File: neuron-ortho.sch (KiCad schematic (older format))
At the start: 138 parts, among them J1 USB_C_Receptacle, J2 Conn_01x04_Male, J3 Conn_01x06_Male, J4 Conn_01x04_Male, J5 Conn_01x04_Male, Q1 DTC123J, SW1 SW_Push, U1 STM32F303C6Tx, U2 NCP1117-3.3_SOT223, U3 USBLC6-2SC6, Y1 8MHz

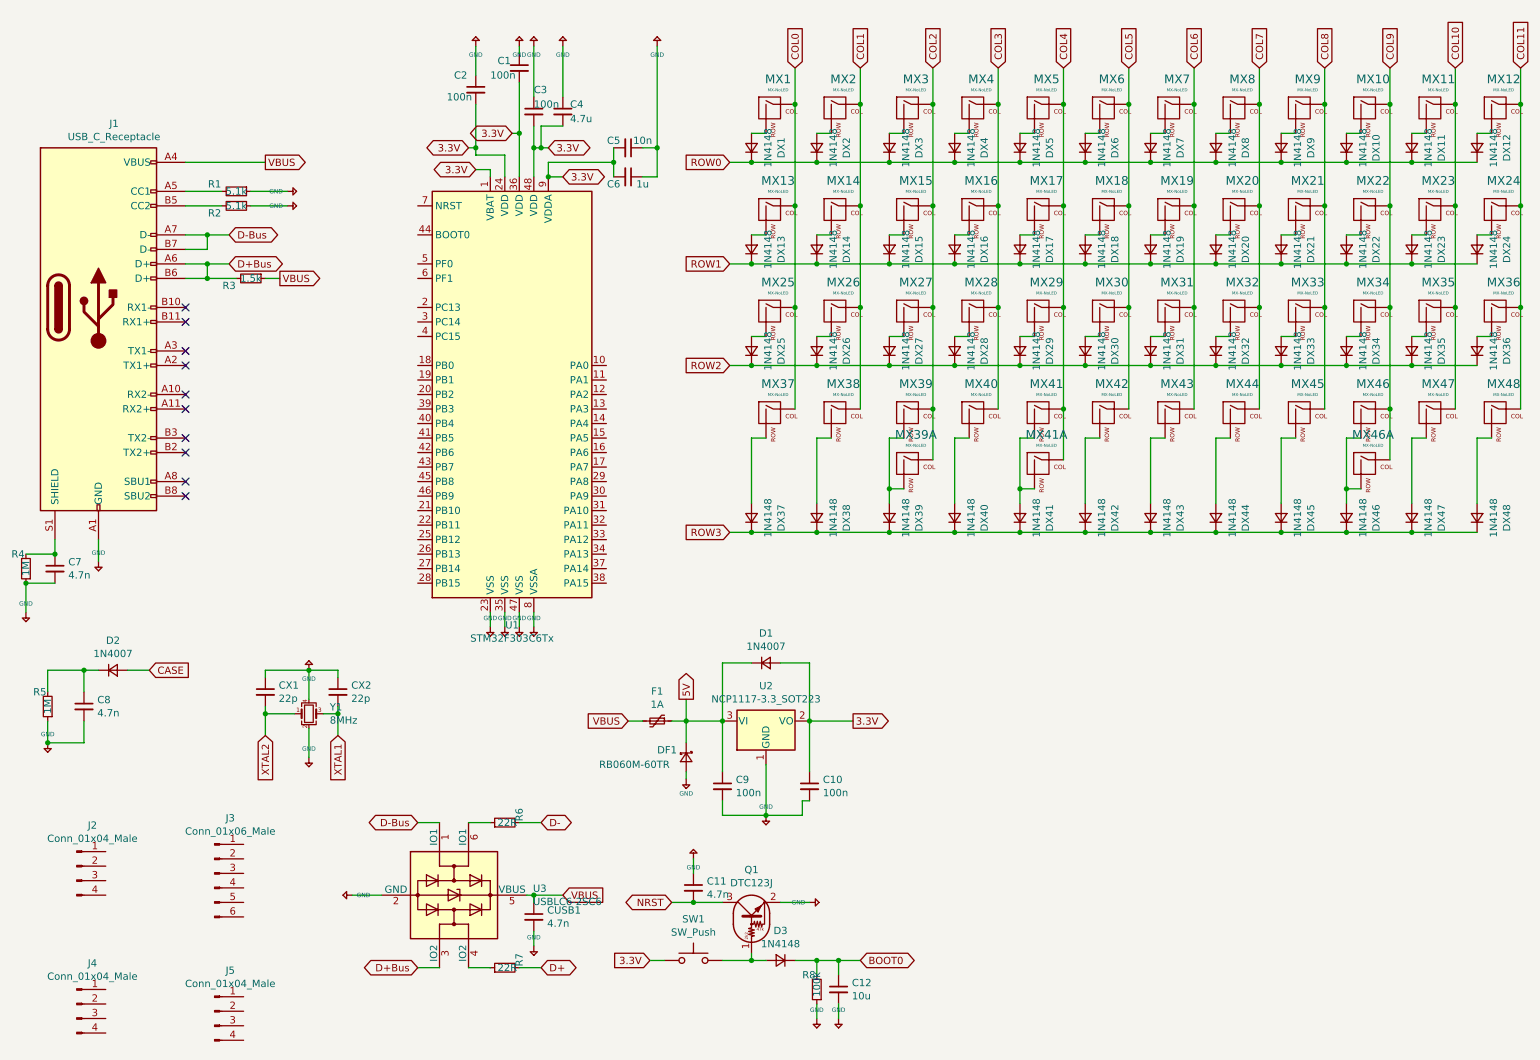
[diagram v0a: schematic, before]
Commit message: Assigned some MCU pins
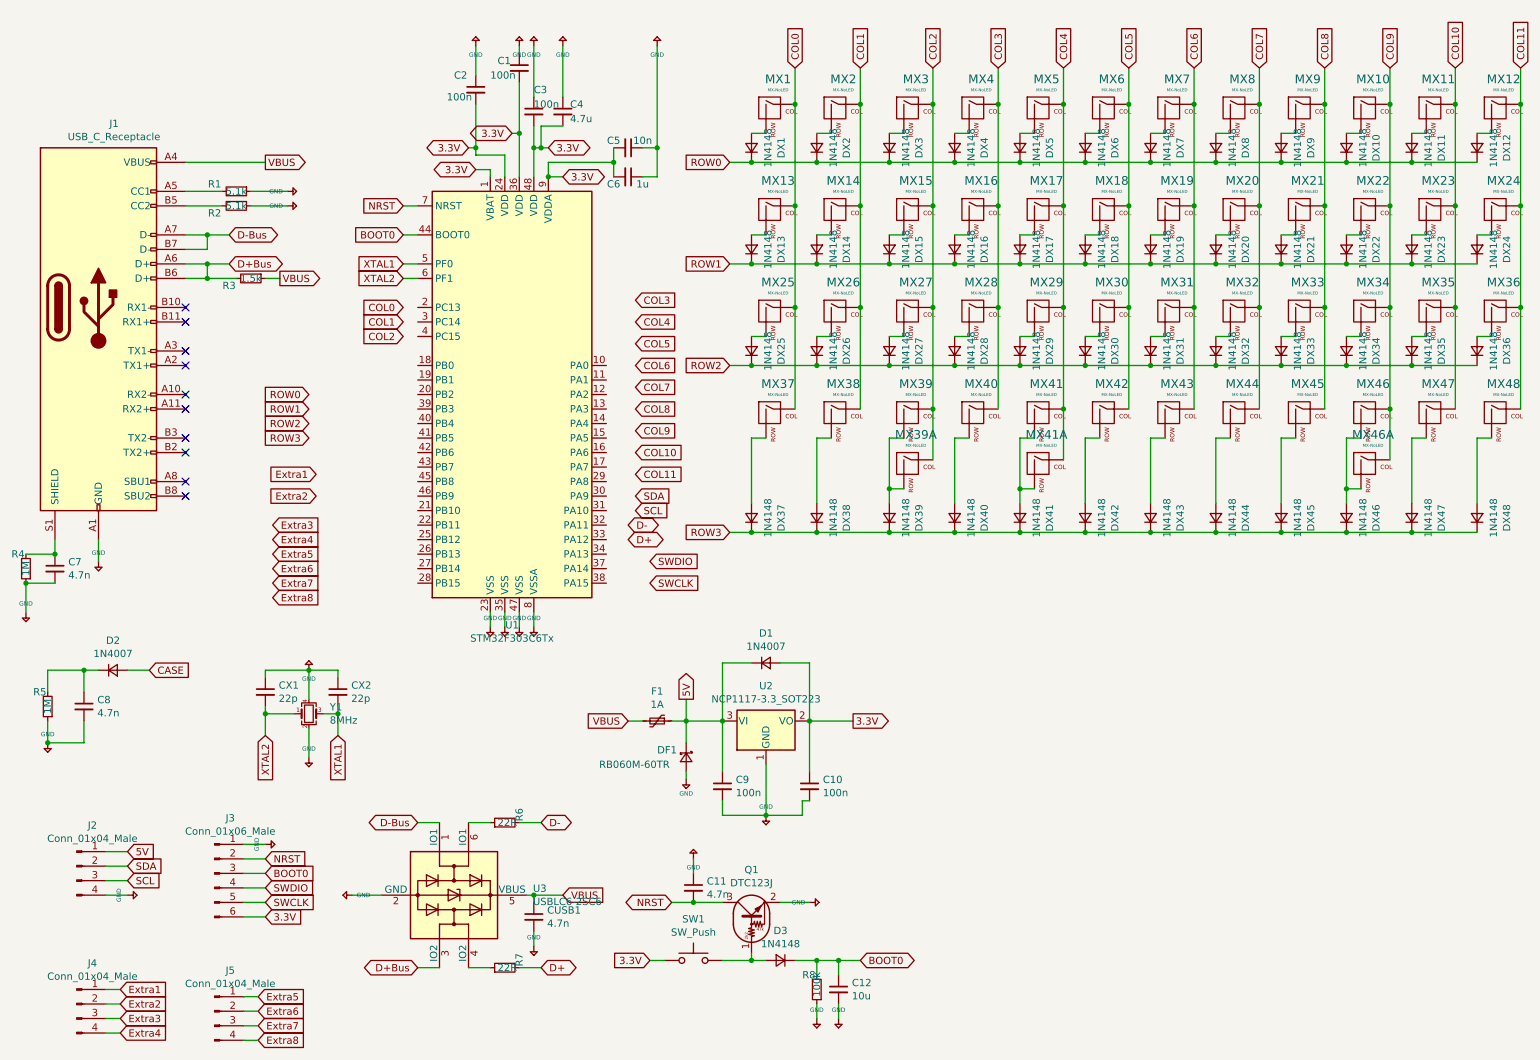
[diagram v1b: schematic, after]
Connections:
- net +5V: now also J2.4 (Pin_4), J3.1 (Pin_1)
- net 3.3V: now also J3.6 (Pin_6)
- net 5V: now also J2.1 (Pin_1)
- net BOOT0: now also J3.3 (Pin_3), U1.44 (BOOT0)
- net NRST: now also J3.2 (Pin_2), U1.7 (NRST)
- net XTAL1: now also U1.5 (PF0)
- net XTAL2: now also U1.6 (PF1)
- net SDA: now reaches J2.2 (Pin_2)
- net SCL: now reaches J2.3 (Pin_3)
- net SWDIO: now reaches J3.4 (Pin_4)
- net SWCLK: now reaches J3.5 (Pin_5)
- net Extra1: now reaches J4.1 (Pin_1)
- net Extra2: now reaches J4.2 (Pin_2)
- net Extra3: now reaches J4.3 (Pin_3)
- net Extra4: now reaches J4.4 (Pin_4)
- net Extra5: now reaches J5.1 (Pin_1)
- net Extra6: now reaches J5.2 (Pin_2)
- net Extra7: now reaches J5.3 (Pin_3)
- net Extra8: now reaches J5.4 (Pin_4)
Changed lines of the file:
@@
 Wire Wire Line
 	6600 2700 6700 2700
+Text GLabel 3250 1800 0    50   Input ~ 0
+NRST
+Wire Wire Line
+	3350 1800 3250 1800
+Wire Wire Line
+	3250 2000 3350 2000
+Text GLabel 3250 2200 0    50   Input ~ 0
+XTAL1
+Text GLabel 3250 2300 0    50   Input ~ 0
+XTAL2
+Wire Wire Line
+	3250 2200 3350 2200
+Wire Wire Line
+	3350 2300 3250 2300
+Text GLabel 4800 4000 2    50   BiDi ~ 0
+D-
+Text GLabel 4800 4100 2    50   BiDi ~ 0
+D+
+Text GLabel 3250 2500 0    50   Input ~ 0
+COL0
+Text GLabel 3250 2600 0    50   Input ~ 0
+COL1
+Text GLabel 3250 2700 0    50   Input ~ 0
+COL2
+Text GLabel 2600 3100 0    50   Input ~ 0
+ROW0
+Text GLabel 2600 3200 0    50   Input ~ 0
+ROW1
+Text GLabel 2600 3300 0    50   Input ~ 0
+ROW2
+Text GLabel 2600 3400 0    50   Input ~ 0
+ROW3
+Text GLabel 4850 2450 2    50   Input ~ 0
+COL3
+Text GLabel 4850 2600 2    50   Input ~ 0
+COL4
+Text GLabel 4850 2750 2    50   Input ~ 0
+COL5
+Text GLabel 4850 2900 2    50   Input ~ 0
+COL6
+Text GLabel 4850 3050 2    50   Input ~ 0
+COL7
+Text GLabel 4850 3200 2    50   Input ~ 0
+COL8
+Text GLabel 4850 3350 2    50   Input ~ 0
+COL9
+Text GLabel 4850 3500 2    50   Input ~ 0
+COL10
+Text GLabel 4850 3650 2    50   Input ~ 0
+COL11
+$Comp
+L keyboard_parts:GND #PWR?
+U 1 1 5E796914
+P 1350 6550
+F 0 "#PWR?" H 1350 6600 20  0001 C CNN
+F 1 "GND" H 1350 6609 30  0000 C CNN
+F 2 "" H 1350 6550 60  0000 C CNN
+F 3 "" H 1350 6550 60  0000 C CNN
+	1    1350 6550
+	0    -1   -1   0
+$EndComp
+$Comp
+L keyboard_parts:GND #PWR?
+U 1 1 5E79741B
+P 2300 6200
+F 0 "#PWR?" H 2300 6250 20  0001 C CNN
+F 1 "GND" H 2300 6259 30  0000 C CNN
+F 2 "" H 2300 6200 60  0000 C CNN
+F 3 "" H 2300 6200 60  0000 C CNN
+	1    2300 6200
+	0    -1   -1   0
+$EndComp
+Text GLabel 1350 6250 2    50   Input ~ 0
+5V
+Text GLabel 1350 6350 2    50   Input ~ 0
+SDA
+Text GLabel 1350 6450 2    50   Input ~ 0
+SCL
+Text GLabel 2300 6300 2    50   Input ~ 0
+NRST
+Text GLabel 2300 6400 2    50   Input ~ 0
+BOOT0
+Text GLabel 2300 6500 2    50   Input ~ 0
+SWDIO
+Text GLabel 2300 6600 2    50   Input ~ 0
+SWCLK
+Text GLabel 2300 6700 2    50   Input ~ 0
+3.3V
+Text GLabel 2250 7250 2    50   Input ~ 0
+Extra5
+Text GLabel 2250 7350 2    50   Input ~ 0
+Extra6
+Text GLabel 2250 7450 2    50   Input ~ 0
+Extra7
+Text GLabel 2250 7550 2    50   Input ~ 0
+Extra8
+Text GLabel 1300 7200 2    50   Input ~ 0
+Extra1
+Text GLabel 1300 7300 2    50   Input ~ 0
+Extra2
+Text GLabel 1300 7400 2    50   Input ~ 0
+Extra3
+Text GLabel 1300 7500 2    50   Input ~ 0
+Extra4
+Wire Wire Line
+	1200 6250 1350 6250
+Wire Wire Line
+	1200 6350 1350 6350
+Wire Wire Line
+	1200 6450 1350 6450
+Wire Wire Line
+	1200 6550 1350 6550
+Wire Wire Line
+	2150 6200 2300 6200
+Wire Wire Line
+	2150 6300 2300 6300
+Wire Wire Line
+	2150 6400 2300 6400
+Wire Wire Line
+	2150 6500 2300 6500
+Wire Wire Line
+	2150 6600 2300 6600
+Wire Wire Line
+	2150 6700 2300 6700
+Wire Wire Line
+	1200 7200 1300 7200
+Wire Wire Line
+	1200 7300 1300 7300
+Wire Wire Line
+	1200 7400 1300 7400
+Wire Wire Line
+	1200 7500 1300 7500
+Wire Wire Line
+	2150 7250 2250 7250
+Wire Wire Line
+	2150 7350 2250 7350
+Wire Wire Line
+	2150 7450 2250 7450
+Wire Wire Line
+	2150 7550 2250 7550
+Text GLabel 3250 2000 0    50   Input ~ 0
+BOOT0
+Text GLabel 4950 4250 2    50   Input ~ 0
+SWDIO
+Text GLabel 4950 4400 2    50   Input ~ 0
+SWCLK
+Text GLabel 4850 3800 2    50   Input ~ 0
+SDA
+Text GLabel 4850 3900 2    50   Input ~ 0
+SCL
+Text GLabel 2650 3650 0    50   Input ~ 0
+Extra1
+Text GLabel 2650 3800 0    50   Input ~ 0
+Extra2
+Text GLabel 2350 4000 2    50   Input ~ 0
+Extra3
+Text GLabel 2350 4100 2    50   Input ~ 0
+Extra4
+Text GLabel 2350 4200 2    50   Input ~ 0
+Extra5
+Text GLabel 2350 4300 2    50   Input ~ 0
+Extra6
+Text GLabel 2350 4400 2    50   Input ~ 0
+Extra7
+Text GLabel 2350 4500 2    50   Input ~ 0
+Extra8
 $EndSCHEMATC
